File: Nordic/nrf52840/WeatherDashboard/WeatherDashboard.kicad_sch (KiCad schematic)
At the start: 0 parts

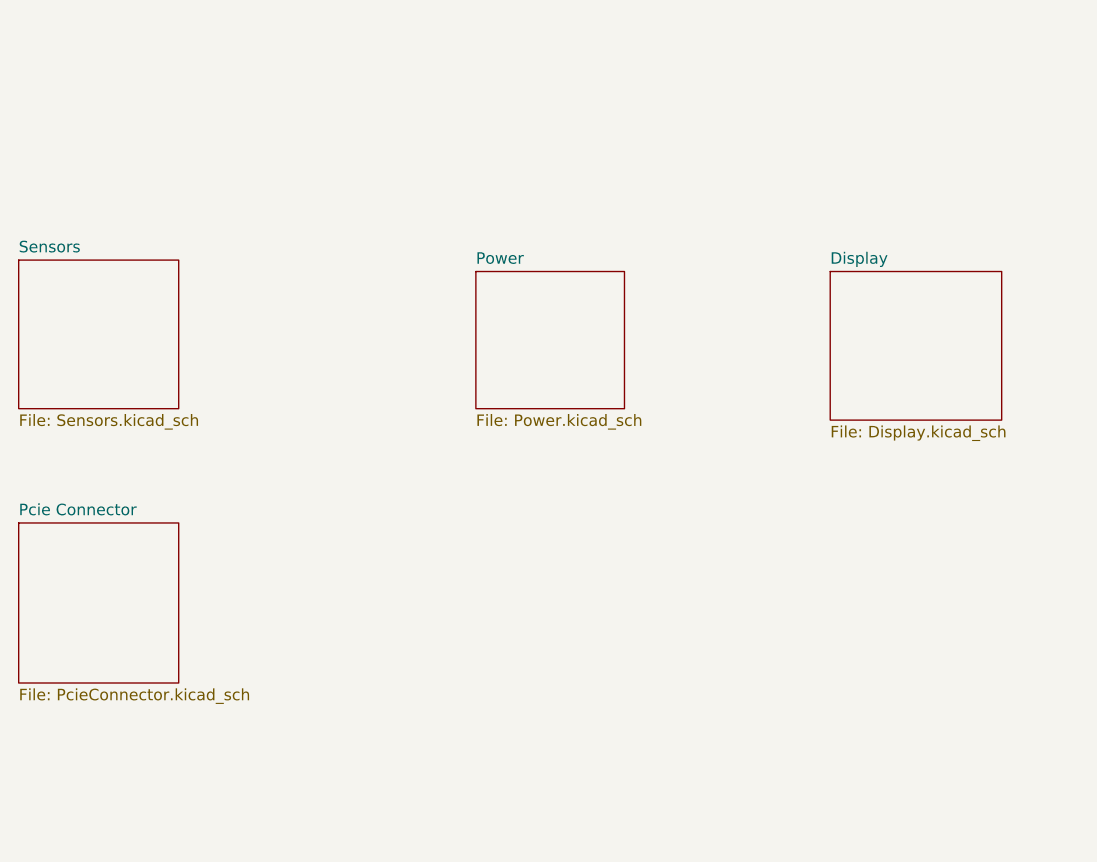
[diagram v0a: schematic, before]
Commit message: pcie connector
Add connectins to the pcie connector
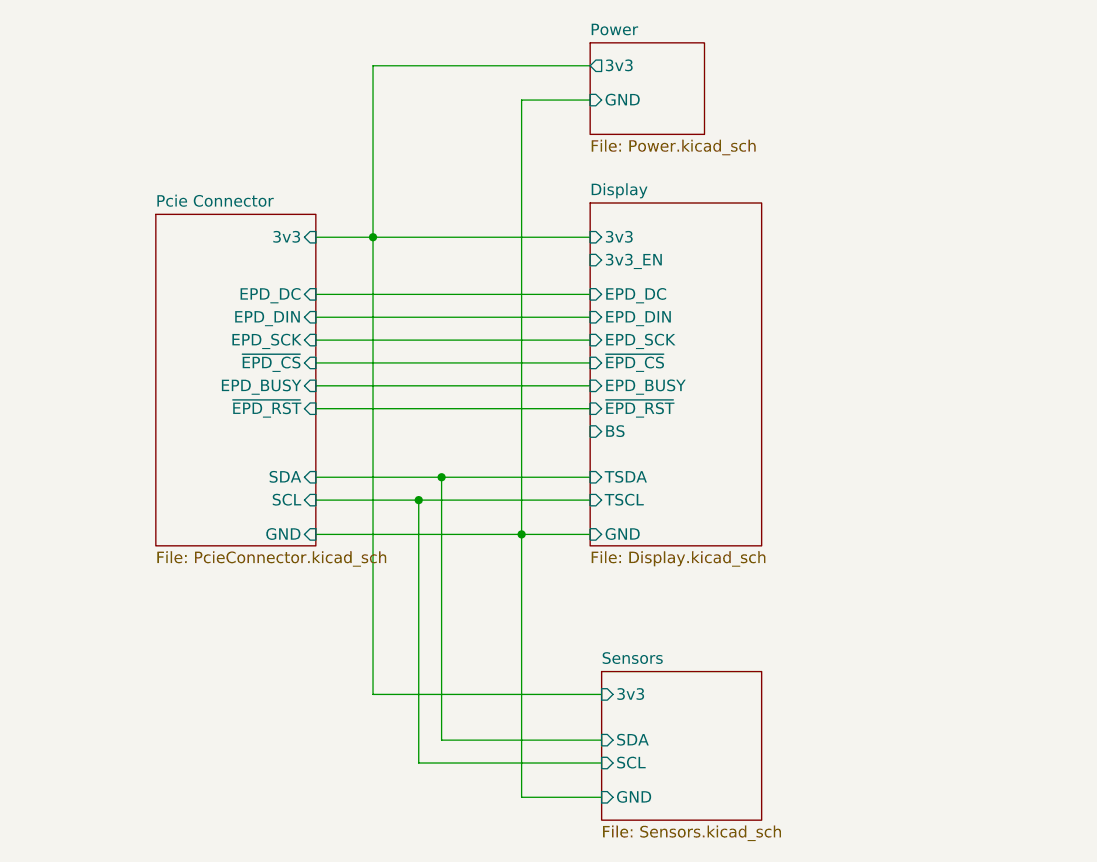
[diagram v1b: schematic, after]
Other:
- sheet Display ports: added 3v3, 3v3_EN, BS, EPD_BUSY, EPD_DC, EPD_DIN, EPD_SCK, GND, TSCL, TSDA, ~{EPD_CS}, ~{EPD_RST}; removed none
- sheet Pcie Connector ports: added 3v3, EPD_BUSY, EPD_DC, EPD_DIN, EPD_SCK, GND, SCL, SDA, ~{EPD_CS}, ~{EPD_RST}; removed none
- sheet Power ports: added 3v3, GND; removed none
- sheet Sensors ports: added 3v3, GND, SCL, SDA; removed none
